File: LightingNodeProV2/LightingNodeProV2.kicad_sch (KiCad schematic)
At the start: 4 parts, among them J1 sata15, J2 Conn_01x03, J3 Conn_01x03, U1 ProMicro_ProMicro

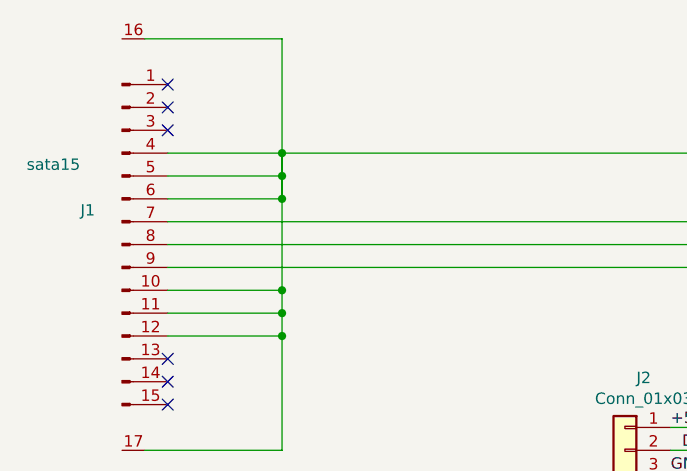
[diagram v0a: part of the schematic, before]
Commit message: edit
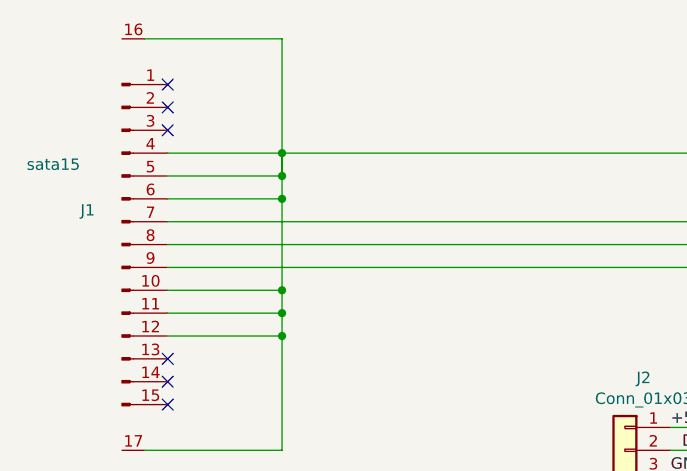
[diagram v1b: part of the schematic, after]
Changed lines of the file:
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@@
-    (stroke (width 0) (type default) (color 0 0 0 1))
-  )
-  (wire (pts (xy 48.26 40.64) (xy 48.26 43.18))
     (stroke (width 0) (type default) (color 0 0 0 1))
   )
